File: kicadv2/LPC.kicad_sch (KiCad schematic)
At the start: 6 parts, among them J2 USB_B_Micro, J7 Conn_01x01_Female, J8 Conn_01x01_Female, J9 Conn_01x01_Female

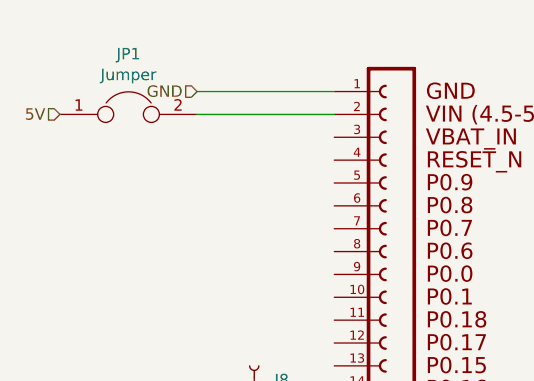
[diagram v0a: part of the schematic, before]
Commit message: simulaciones y kicad para placa nueva
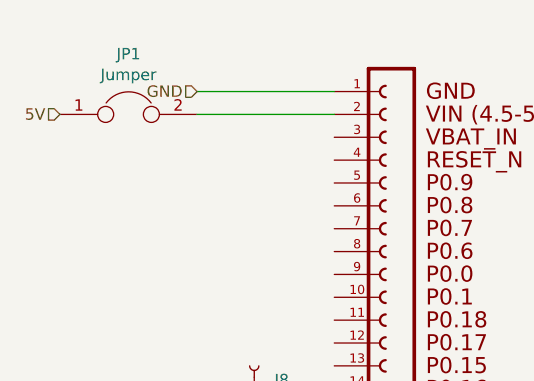
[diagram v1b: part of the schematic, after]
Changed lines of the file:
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@@
     (effects (font (size 1.27 1.27)) (justify right))
   )
-  (symbol (lib_id "potenciostato-rescue:LPCXPRESSO_LPC1769-LPCXPRESSO_LPC1769") (at 101.6 78.74 0) (unit 1)
+  (symbol (lib_id "potenciostato-rescue:LPCXPRESSO_LPC1769-LPCXPRESSO_LPC1769") (at 101.6 78.74 0)
     (in_bom yes) (on_board yes)
     (property "Reference" "LPC1" (id 0) (at 105.41 36.322 0))
@@
     (pin "9")
   )
-  (symbol (lib_id "potenciostato-rescue:USB_B_Micro-Connector") (at 173.99 66.04 180) (unit 1)
+  (symbol (lib_id "potenciostato-rescue:USB_B_Micro-Connector") (at 173.99 66.04 180)
     (in_bom yes) (on_board yes)
     (property "Reference" "J2" (id 0) (at 179.832 63.3984 0)
